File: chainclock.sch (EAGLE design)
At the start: 21 parts, among them SW1 ROTARTY_ENCODER

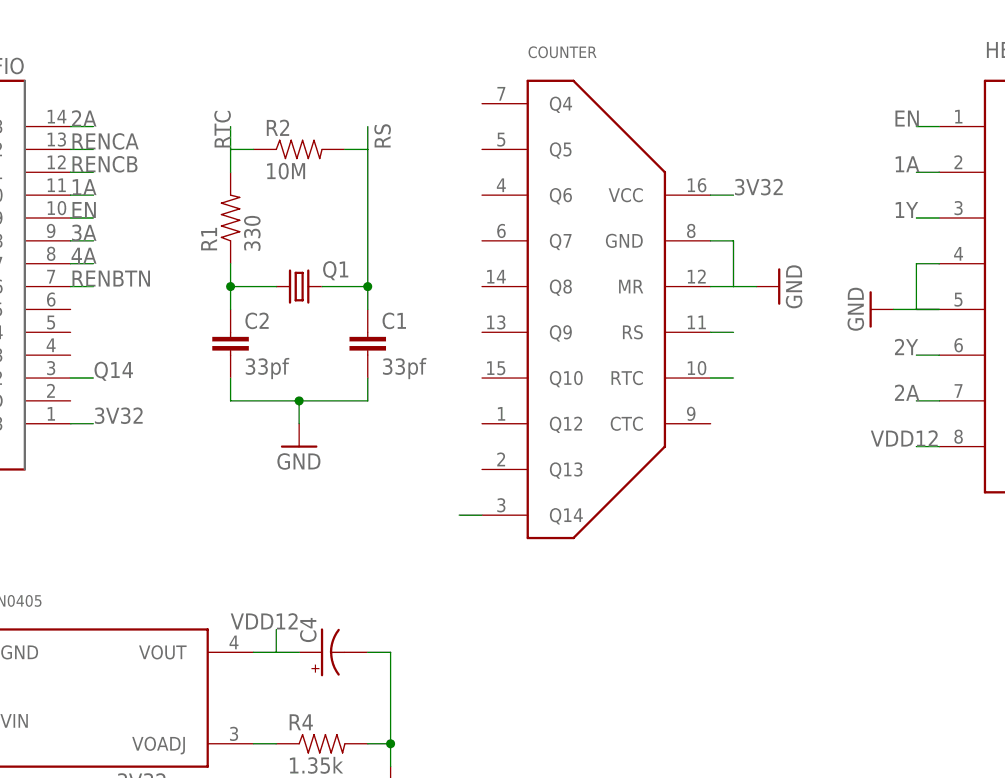
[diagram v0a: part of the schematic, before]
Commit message: Switch out crystal
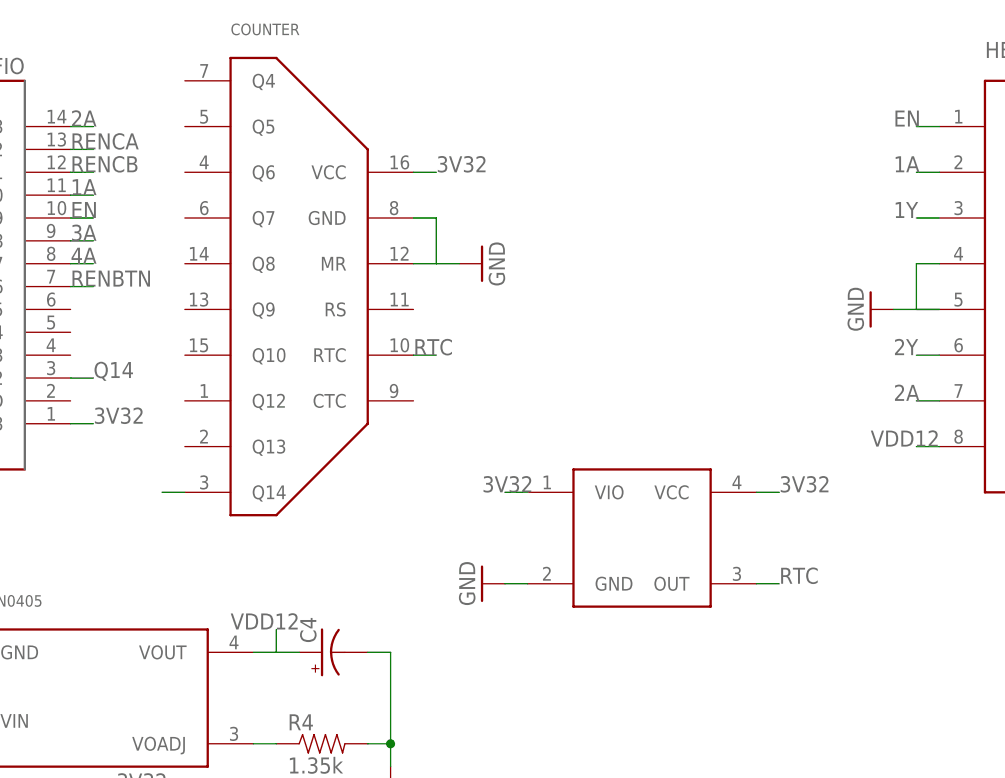
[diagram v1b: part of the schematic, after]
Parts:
- removed C1, C2: 33pf, SparkFun-Capacitors:0.1UF-50V-20%(PTH)KIT-EZ
- removed Q1: (no value), adafruit:CRYSTALTC26H
- removed R1: 330, SparkFun-Resistors:RESISTOREZ
- removed R2: 10M, SparkFun-Resistors:RESISTOREZ
- added U$4: SG30XXJC, desjardins:SG30XXJC
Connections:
- removed net N$1: C2.1, Q1.1, R1.1
- removed net RS: C1.1, COUNTER.RS, Q1.2, R2.2
- net 3V32: now also U$4.VCC, U$4.VIO
- net GND: now also U$4.GND; no longer C1.2, C2.2
- net RTC: now also U$4.OUT; no longer R1.2, R2.1
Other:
- moved on the sheet: COUNTER
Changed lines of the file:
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@@
 <part name="COUNTER" library="desjardins" deviceset="4060" device=""/>
 <part name="ARDUNOFIO" library="desjardins" deviceset="ARDUINOFIO" device=""/>
-<part name="R1" library="SparkFun-Resistors" deviceset="RESISTOR" device="EZ" value="330"/>
-<part name="R2" library="SparkFun-Resistors" deviceset="RESISTOR" device="EZ" value="10M"/>
-<part name="C1" library="SparkFun-Capacitors" deviceset="0.1UF-50V-20%(PTH)" device="KIT-EZ" value="33pf"/>
-<part name="C2" library="SparkFun-Capacitors" deviceset="0.1UF-50V-20%(PTH)" device="KIT-EZ" value="33pf"/>
-<part name="Q1" library="adafruit" deviceset="CRYSTAL" device="TC26H"/>
-<part name="GND1" library="SparkFun-Aesthetics" deviceset="GND" device=""/>
 <part name="HBRIDGE" library="desjardins" deviceset="SN754410" device=""/>
 <part name="GND2" library="SparkFun-Aesthetics" deviceset="GND" device=""/>
@@
 <part name="R5" library="SparkFun-Resistors" deviceset="RESISTOR" device="2010" value="10k"/>
 <part name="R6" library="SparkFun-Resistors" deviceset="RESISTOR" device="2010" value="10k"/>
+<part name="GND1" library="SparkFun-Aesthetics" deviceset="GND" device=""/>
+<part name="U$4" library="desjardins" deviceset="SG30XX" device="JC"/>
 </parts>
 <sheets>
@@
 </plain>
 <instances>
-<instance part="COUNTER" gate="G$1" x="101.6" y="180.34"/>
+<instance part="COUNTER" gate="G$1" x="68.58" y="182.88"/>
 <instance part="ARDUNOFIO" gate="G$1" x="27.94" y="182.88" rot="R90"/>
-<instance part="R1" gate="G$1" x="60.96" y="190.5" rot="R90"/>
-<instance part="R2" gate="G$1" x="68.58" y="198.12"/>
-<instance part="C1" gate="G$1" x="76.2" y="175.26"/>
-<instance part="C2" gate="G$1" x="60.96" y="175.26"/>
-<instance part="Q1" gate="G$1" x="68.58" y="182.88"/>
-<instance part="GND1" gate="1" x="68.58" y="165.1"/>
 <instance part="HBRIDGE" gate="G$1" x="154.94" y="177.8"/>
-<instance part="GND2" gate="1" x="121.92" y="182.88" rot="R90"/>
+<instance part="GND2" gate="1" x="88.9" y="185.42" rot="R90"/>
 <instance part="GND3" gate="1" x="132.08" y="180.34" rot="R270"/>
 <instance part="GND4" gate="1" x="177.8" y="180.34" rot="R90"/>
@@
 <instance part="R5" gate="G$1" x="83.82" y="96.52" rot="MR180"/>
 <instance part="R6" gate="G$1" x="58.42" y="96.52" rot="MR180"/>
+<instance part="GND1" gate="1" x="88.9" y="149.86" rot="R270"/>
+<instance part="U$4" gate="G$1" x="106.68" y="154.94"/>
 </instances>
 <busses>
@@
 <net name="GND" class="0">
 <segment>
-<pinref part="C2" gate="G$1" pin="2"/>
-<wire x1="60.96" y1="172.72" x2="60.96" y2="170.18" width="0.1524" layer="91"/>
-<pinref part="C1" gate="G$1" pin="2"/>
-<wire x1="76.2" y1="172.72" x2="76.2" y2="170.18" width="0.1524" layer="91"/>
-<wire x1="60.96" y1="170.18" x2="68.58" y2="170.18" width="0.1524" layer="91"/>
-<wire x1="76.2" y1="170.18" x2="68.58" y2="170.18" width="0.1524" layer="91"/>
-<wire x1="68.58" y1="170.18" x2="68.58" y2="167.64" width="0.1524" layer="91"/>
-<junction x="68.58" y="170.18"/>
-<pinref part="GND1" gate="1" pin="GND"/>
-</segment>
-<segment>
 <pinref part="COUNTER" gate="G$1" pin="GND"/>
-<wire x1="114.3" y1="187.96" x2="116.84" y2="187.96" width="0.1524" layer="91"/>
+<wire x1="81.28" y1="190.5" x2="83.82" y2="190.5" width="0.1524" layer="91"/>
 <pinref part="COUNTER" gate="G$1" pin="MR"/>
-<wire x1="114.3" y1="182.88" x2="116.84" y2="182.88" width="0.1524" layer="91"/>
-<wire x1="116.84" y1="187.96" x2="116.84" y2="182.88" width="0.1524" layer="91"/>
-<wire x1="116.84" y1="182.88" x2="119.38" y2="182.88" width="0.1524" layer="91"/>
+<wire x1="81.28" y1="185.42" x2="83.82" y2="185.42" width="0.1524" layer="91"/>
+<wire x1="83.82" y1="190.5" x2="83.82" y2="185.42" width="0.1524" layer="91"/>
+<wire x1="83.82" y1="185.42" x2="86.36" y2="185.42" width="0.1524" layer="91"/>
 <pinref part="GND2" gate="1" pin="GND"/>
 </segment>
@@
 <pinref part="GND12" gate="1" pin="GND"/>
 </segment>
-</net>
-<net name="N$1" class="0">
-<segment>
-<pinref part="Q1" gate="G$1" pin="1"/>
-<wire x1="66.04" y1="182.88" x2="60.96" y2="182.88" width="0.1524" layer="91"/>
-<pinref part="C2" gate="G$1" pin="1"/>
-<wire x1="60.96" y1="182.88" x2="60.96" y2="180.34" width="0.1524" layer="91"/>
-<wire x1="60.96" y1="182.88" x2="60.96" y2="185.42" width="0.1524" layer="91"/>
-<pinref part="R1" gate="G$1" pin="1"/>
-<junction x="60.96" y="182.88"/>
-</segment>
-</net>
-<net name="RS" class="0">
-<segment>
-<pinref part="Q1" gate="G$1" pin="2"/>
-<wire x1="71.12" y1="182.88" x2="76.2" y2="182.88" width="0.1524" layer="91"/>
-<pinref part="C1" gate="G$1" pin="1"/>
-<wire x1="76.2" y1="182.88" x2="76.2" y2="180.34" width="0.1524" layer="91"/>
-<wire x1="76.2" y1="182.88" x2="76.2" y2="198.12" width="0.1524" layer="91"/>
-<pinref part="R2" gate="G$1" pin="2"/>
-<wire x1="76.2" y1="198.12" x2="73.66" y2="198.12" width="0.1524" layer="91"/>
-<junction x="76.2" y="182.88"/>
-<wire x1="76.2" y1="198.12" x2="76.2" y2="200.66" width="0.1524" layer="91"/>
-<label x="78.74" y="198.12" size="1.778" layer="95" rot="R90"/>
-</segment>
-<segment>
-<pinref part="COUNTER" gate="G$1" pin="RS"/>
-<wire x1="114.3" y1="177.8" x2="116.84" y2="177.8" width="0.1524" layer="91"/>
-</segment>
-</net>
-<net name="RTC" class="0">
-<segment>
-<pinref part="R1" gate="G$1" pin="2"/>
-<wire x1="60.96" y1="195.58" x2="60.96" y2="198.12" width="0.1524" layer="91"/>
-<wire x1="60.96" y1="198.12" x2="63.5" y2="198.12" width="0.1524" layer="91"/>
-<pinref part="R2" gate="G$1" pin="1"/>
-<wire x1="60.96" y1="198.12" x2="60.96" y2="200.66" width="0.1524" layer="91"/>
-<label x="60.96" y="198.12" size="1.778" layer="95" rot="R90"/>
-</segment>
-<segment>
-<pinref part="COUNTER" gate="G$1" pin="RTC"/>
-<wire x1="114.3" y1="172.72" x2="116.84" y2="172.72" width="0.1524" layer="91"/>
+<segment>
+<wire x1="93.98" y1="149.86" x2="91.44" y2="149.86" width="0.1524" layer="91"/>
+<pinref part="GND1" gate="1" pin="GND"/>
+<pinref part="U$4" gate="G$1" pin="GND"/>
 </segment>
 </net>
@@
 <segment>
 <pinref part="COUNTER" gate="G$1" pin="Q14"/>
-<wire x1="88.9" y1="157.48" x2="86.36" y2="157.48" width="0.1524" layer="91"/>
+<wire x1="55.88" y1="160.02" x2="53.34" y2="160.02" width="0.1524" layer="91"/>
 </segment>
 <segment>
@@
 <segment>
 <pinref part="COUNTER" gate="G$1" pin="VCC"/>
-<wire x1="114.3" y1="193.04" x2="116.84" y2="193.04" width="0.1524" layer="91"/>
-<label x="116.84" y="193.04" size="1.778" layer="95"/>
+<wire x1="81.28" y1="195.58" x2="83.82" y2="195.58" width="0.1524" layer="91"/>
+<label x="83.82" y="195.58" size="1.778" layer="95"/>
 </segment>
 <segment>
@@
 <pinref part="R12" gate="G$1" pin="2"/>
 </segment>
+<segment>
+<wire x1="119.38" y1="160.02" x2="121.92" y2="160.02" width="0.1524" layer="91"/>
+<label x="121.92" y="160.02" size="1.778" layer="95"/>
+<pinref part="U$4" gate="G$1" pin="VCC"/>
+</segment>
+<segment>
+<wire x1="93.98" y1="160.02" x2="91.44" y2="160.02" width="0.1524" layer="91"/>
+<label x="88.9" y="160.02" size="1.778" layer="95"/>
+<pinref part="U$4" gate="G$1" pin="VIO"/>
+</segment>
 </net>
 <net name="VDD12" class="0">
@@
 </segment>
 </net>
+<net name="RTC" class="0">
+<segment>
+<pinref part="COUNTER" gate="G$1" pin="RTC"/>
+<wire x1="81.28" y1="175.26" x2="83.82" y2="175.26" width="0.1524" layer="91"/>
+<label x="81.28" y="175.26" size="1.778" layer="95"/>
+</segment>
+<segment>
+<wire x1="119.38" y1="149.86" x2="121.92" y2="149.86" width="0.1524" layer="91"/>
+<label x="121.92" y="149.86" size="1.778" layer="95"/>
+<pinref part="U$4" gate="G$1" pin="OUT"/>
+</segment>
+</net>
